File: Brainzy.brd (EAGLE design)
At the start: 80 x 75 mm, 74 parts, among them J7 5.5x2.1mm Barrel, Q1 BSS138, Q2 BSS138, Q3 BSS138, Q4 BSS138, T1 BSS84, T2 BSS84, T3 BSS84, T4 SI2323DS, U1 L293DD, U2 L293DD, U3 HC_05, U4 GY-521MPU6050

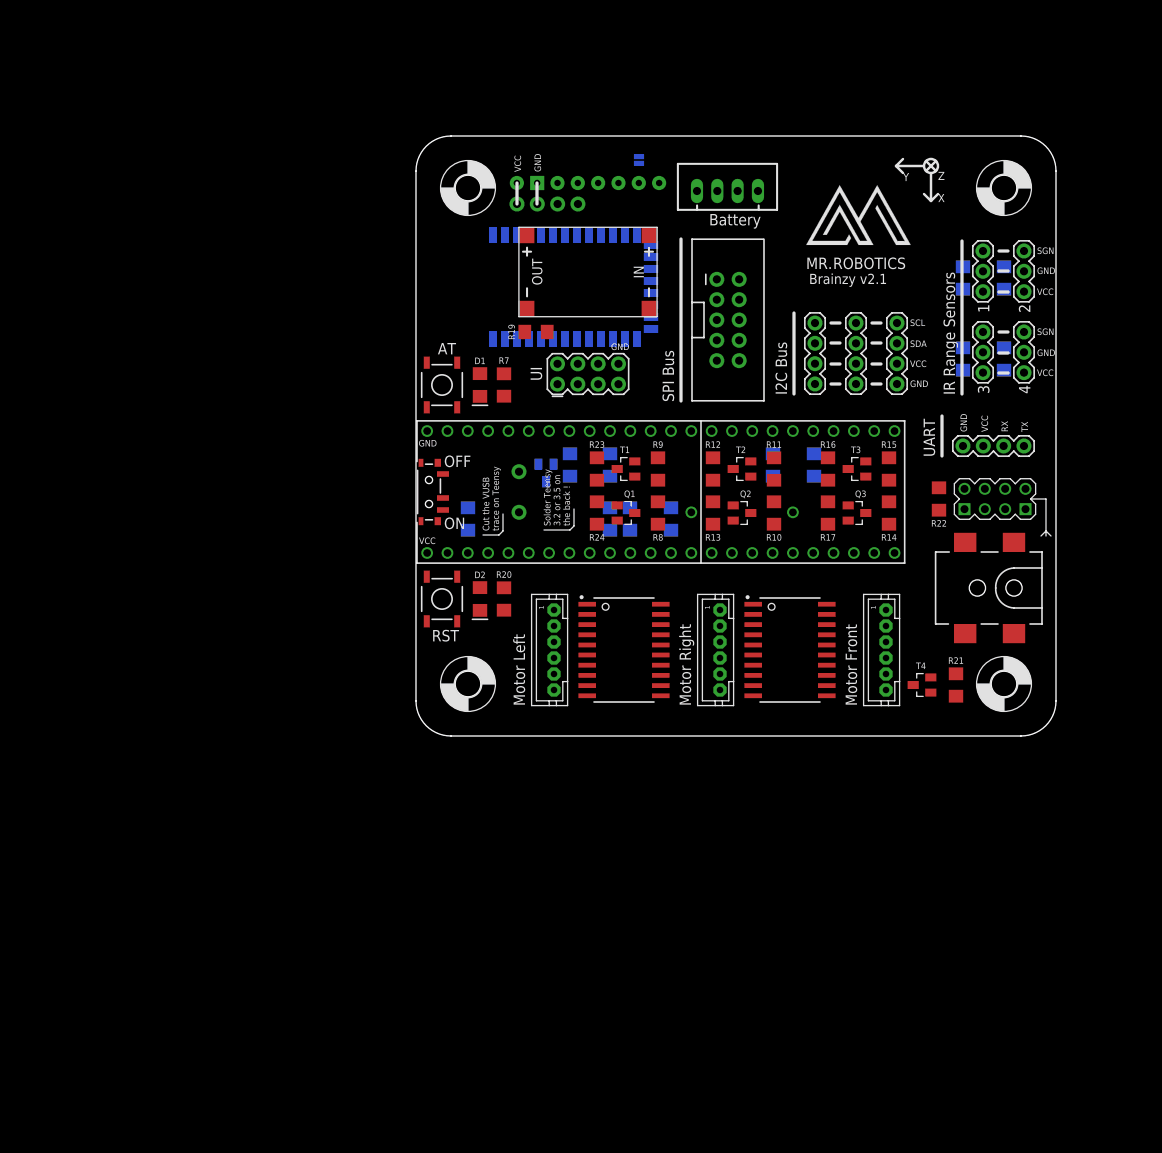
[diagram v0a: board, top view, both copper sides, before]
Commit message: Upload Brainzy v3.0
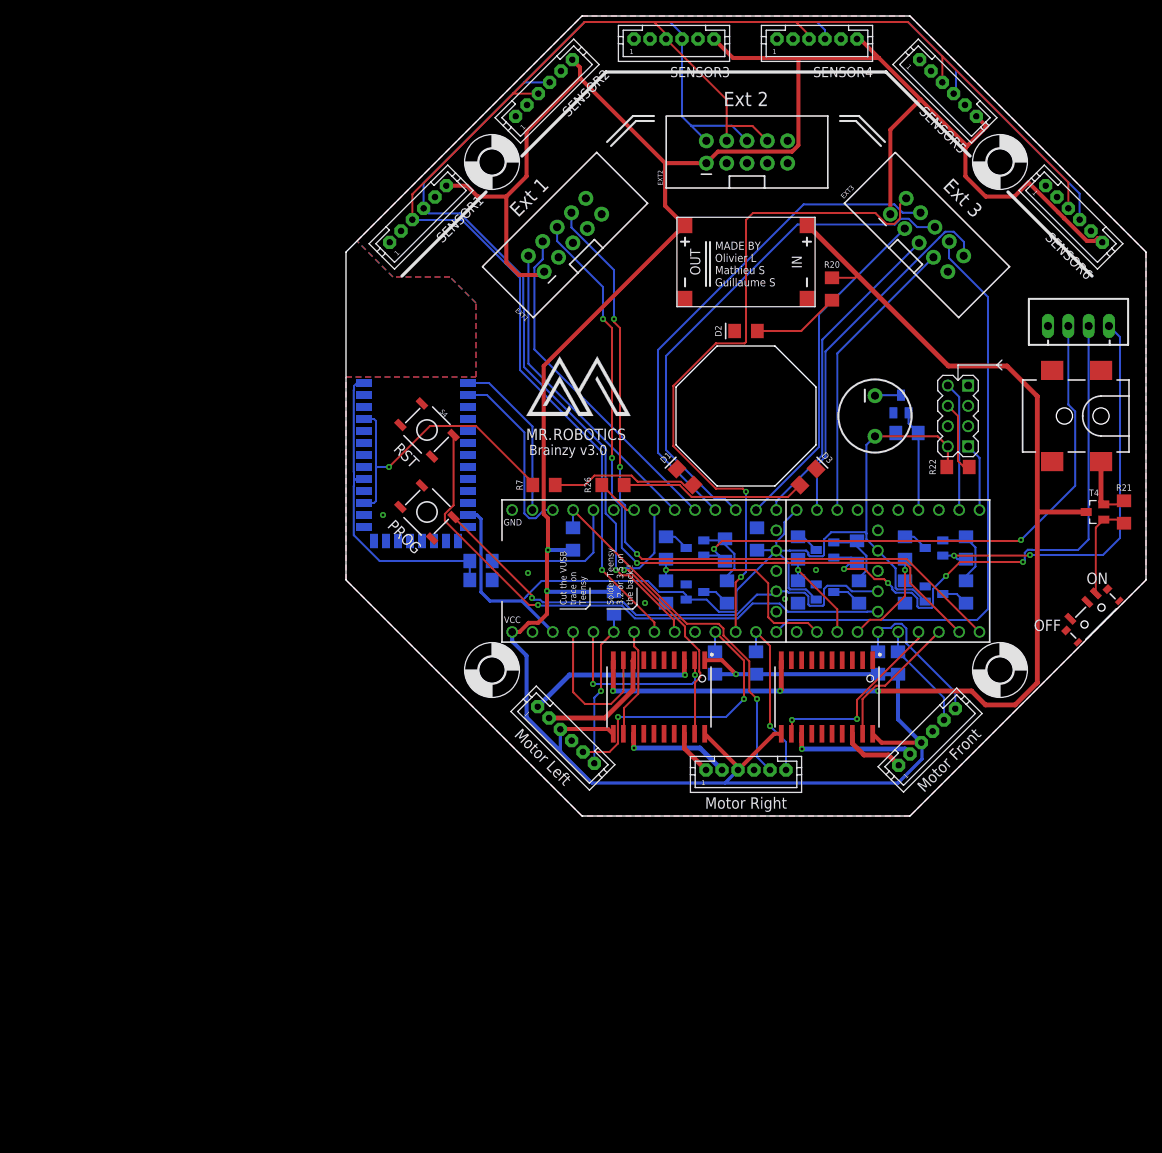
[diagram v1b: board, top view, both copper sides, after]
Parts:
- removed C1, C2, C3, C4: 10uF, SparkFun-Capacitors:1206
- removed EXT_BT: (no value), SparkFun-Connectors:1X04_NO_SILK
- removed H1, H2, H3, H4: MOUNT-HOLE3.2, holes:3,2
- removed I2C1, I2C2, I2C3, UART: (no value), SparkFun-Connectors:1X04
- removed JP1: JUMPER-SMT_2_NO_NO-SILK, SparkFun-Jumpers:SMT-JUMPER_2_NO_NO-SILK
- removed S1: (no value), SparkFun-Switches:TACTILE_SWITCH_SMD_5.2MM
- removed SHARP1, SHARP2, SHARP3, SHARP4: (no value), SparkFun-Connectors:1X03
- removed SPI: (no value), MrRobotics-Connectors:2X5-SHROUDED_LOCK
- removed U$4: LOGO_FR, MrRobotics-Aesthetics:LOGO_FR
- removed U4: GY-521MPU6050, MrRobotics-Modules:GY-521
- removed UI: (no value), SparkFun-Connectors:2X4
- added D3: (no value), SparkFun-LED:FKIT-LED-1206
- added EXT1, EXT2, EXT3: (no value), SparkFun-Connectors:2X5-SHROUDED_LOCK
- added R26, R27: 470, SparkFun-Resistors:1206
- added S4: (no value), SparkFun-Switches:TACTILE_SWITCH_SMD_5.2MM
- added SENSOR1, SENSOR2, SENSOR3, SENSOR4, SENSOR5, SENSOR6: (no value), MrRobotics-Connectors:JST-PH6
- added U$10, U$11, U$8, U$9: (no value), holes:3,3
- added U$12: (no value), MrRobotics-Aesthetics:LOGO_M
- added U$5: (no value), MrRobotics-Aesthetics:M_50MM
- R23: value 470k -> 150k
- R24: value 150k -> 470k
- R7: value 750 -> 470
- U$3: value LOGO -> (none); device MrRobotics-Aesthetics:LOGO_M -> MrRobotics-Aesthetics:LOGO_FR
- U$7: device MrRobotics-Aesthetics:LOGO_BACK_NAME -> MrRobotics-Aesthetics:NAME_50MM
- moved S2 84.4 mm to (84.6, 15.0), turned to 225 degrees
- moved U$3 64.6 mm to (28.1, 0.12), flipped to the bottom
- moved R20 56.4 mm to (52.0, 55.9), turned to 90 degrees
- moved U$7 53.0 mm to (65.8, 51.0)
- moved D2 47.2 mm to (41.2, 50.6), turned to 180 degrees
- moved BATT 47.0 mm to (79.0, 51.2)
- moved BUZZER 45.5 mm to (57.4, 40.0), flipped to the top
- moved Q4 45.2 mm to (60.6, 41.5), turned to 0 degrees
- moved R25 42.3 mm to (61.4, 37.9), turned to 0 degrees
- moved R18 36.2 mm to (42.6, 24.6), turned to 270 degrees
- moved R19 31.8 mm to (8.12, 19.5), flipped to the bottom, turned to 180 degrees
- moved R3 30.8 mm to (42.5, 9.12)
- moved T4 30.6 mm to (84.9, 28.0)
- moved R21 30.1 mm to (88.5, 28.0)
- moved D1 28.1 mm to (33.6, 32.4), turned to 135 degrees
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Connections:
- net N$12 renamed PROG
- removed net BTN_CENTER: U$1.4, UI.5
- removed net BTN_DOWN: U$1.7, UI.4
- removed net BTN_LEFT: U$1.3, UI.3
- removed net BTN_RIGHT: U$1.5, UI.6
- removed net BTN_UP: U$1.2, UI.1
- removed net BT_RST: S3.1, U3.11
- removed net DTR: U3.32
- removed net EXT_RX: U$1.31/A12, UART.3
- removed net EXT_TX: U$1.32/A13, UART.4
- removed net MPU_INT: U$1.26, U4.INT
- removed net N$17: JP1.1, U4.ADO
- removed net SHARP1: SHARP1.1, U$1.38/A19
- removed net SHARP2: SHARP2.1, U$1.37/A18
- removed net SHARP3: SHARP3.1, U$1.35/A16
- removed net SHARP4: SHARP4.1, U$1.36/A17
- new net BT_KEY: R27.2, U$1.3
- new net EXT1_RX: EXT1.2, U$1.7
- new net EXT1_TX: EXT1.4, U$1.8
- new net EXT2_RX: EXT1.6, U$1.34/A15
- new net EXT2_TX: EXT1.8, U$1.33/A14
- new net LED_BUILDIN: R26.1, U$1.5
- new net N$12: D3.A, R26.2
- new net RST: S4.2, U$1.RST_3.5
- net 3.3V: now also U$1.3.3V2, U$1.3.3V3; no longer S1.3
- net 5V: now also EXT1.1, EXT2.1, EXT3.1, SENSOR1.6, SENSOR2.6, SENSOR3.6, SENSOR4.6, SENSOR5.6, SENSOR6.6; no longer C1.1, C2.1, C3.1, C4.1, EXT_BT.1, I2C1.2, I2C2.2, I2C3.2, JP1.2, SHARP1.3, SHARP2.3, SHARP3.3, SHARP4.3, SPI.1, U4.VCC, UART.2, UI.2
- net BATT1: now also U$1.A22; no longer U$1.39/A20
- net BATT3: now also U$1.39/A20; no longer U$1.A22
- net BT_RX: no longer EXT_BT.3
- net BT_TX: no longer EXT_BT.4
- net ENC1_B: now also MOT_LEFT.6, R1.1, U$1.21/A7; no longer U$1.17/A3
- net ENC2_A: now also U$1.2; no longer U$1.8
- net ENC2_B: no longer MOT_LEFT.6, R1.1
- net ENC3_A: now also U$1.37/A18; no longer U$1.27
- net ENC3_B: now also U$1.38/A19; no longer U$1.28
- net GND: now also D3.C, EXT1.9, EXT2.9, EXT3.9, S4.4, SENSOR1.1, SENSOR2.1, SENSOR3.1, SENSOR4.1, SENSOR5.1, SENSOR6.1, U$1.GND2, U$1.GND3; no longer C1.2, C2.2, C3.2, C4.2, EXT_BT.2, I2C1.1, I2C2.1, I2C3.1, S3.3, SHARP1.2, SHARP2.2, SHARP3.2, SHARP4.2, SPI.2, U4.GND, UART.1, UI.8
- net I2C_SCL: now also EXT2.4, EXT2.8, SENSOR1.3, SENSOR2.3, SENSOR3.3, SENSOR4.3, SENSOR5.3, SENSOR6.3; no longer I2C1.4, I2C2.4, I2C3.4, U4.SCL
- net I2C_SDA: now also EXT2.2, EXT2.6, SENSOR1.4, SENSOR2.4, SENSOR3.4, SENSOR4.4, SENSOR5.4, SENSOR6.4; no longer I2C1.3, I2C2.3, I2C3.3, U4.SDA
- net MOT1_1: now also U$1.22/A8, U1.2; no longer U$1.23/A9, U1.9
- net MOT1_2: now also U$1.23/A9, U1.9; no longer U$1.22/A8, U1.2
- net MOT1_OUT1: now also U1.3; no longer U1.8
- net MOT1_OUT2: now also U1.8; no longer U1.3
- net MOT2_1: now also U$1.6, U1.19; no longer U$1.21/A7, U1.12
- net MOT2_2: now also U1.12; no longer U1.19
- net MOT2_OUT1: now also U1.18; no longer U1.13
- net MOT2_OUT2: now also U1.13; no longer U1.18
- net MOT3_1: now also U$1.35/A16, U2.19; no longer U$1.29, U2.12
- net MOT3_2: now also U$1.36/A17, U2.12; no longer U$1.30, U2.19
- net MOT3_OUT1: now also U2.18; no longer U2.13
- net MOT3_OUT2: now also U2.13; no longer U2.18
- net N$18: now also R27.1; no longer S1.1
- net N$8: now also U$1.29; no longer U$1.6
- net SPI_CS1: now also EXT3.2; no longer SPI.4
- net SPI_CS2: now also EXT3.4; no longer SPI.6
- net SPI_CS3: now also EXT3.6; no longer SPI.8
- net SPI_MISO: now also EXT3.5; no longer SPI.7
- net SPI_MOSI: now also EXT3.3; no longer SPI.5
- net SPI_SCK: now also EXT3.8; no longer SPI.3
- net T_CS: now also EXT3.7; no longer SPI.9
- net T_IRQ: now also EXT3.10; no longer SPI.10
- net WIFI_RX: now also U$1.31/A12; no longer U$1.34/A15
- net WIFI_TX: now also U$1.32/A13; no longer U$1.33/A14
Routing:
- net 5V: track 0.00 -> 393.6 mm, vias 0 -> 3
- net I2C_SDA: track 0.00 -> 207.7 mm, vias 0 -> 1
- net I2C_SCL: track 0.00 -> 207.0 mm, vias 0 -> 1
- net 12V: track 0.00 -> 145.5 mm, vias 0 -> 3
- net 3.3V: track 0.00 -> 131.1 mm
- net EXT2_TX: track 0.00 -> 92.9 mm, vias 0 -> 3
- net EXT2_RX: track 0.00 -> 91.1 mm, vias 0 -> 3
- net SPI_CS1: track 0.00 -> 86.9 mm, vias 0 -> 2
- net SPI_SCK: track 0.00 -> 75.6 mm
- net S1: track 0.00 -> 73.8 mm, vias 0 -> 2
- net RST: track 0.00 -> 71.6 mm, vias 0 -> 1
- net S2: track 0.00 -> 70.5 mm, vias 0 -> 4
- net SPI_CS3: track 0.00 -> 64.7 mm
- net SPI_CS2: track 0.00 -> 63.8 mm
- net PROG: track 0.00 -> 63.3 mm, vias 0 -> 1
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- added copper zone on layer 1, net GND
- added copper zone on layer 16, net GND
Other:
- board size 80 x 75 mm -> 100 x 100 mm
- board text added: "Brainzy v3.0"
- board text added: "Ext 1"
- board text added: "Ext 2"
- board text added: "Ext 3"
- board text added: "MADE BY Olivier L Mathieu S Guillaume S"
- board text added: "PROG"
- board text removed: "1"
- board text removed: "2"
- board text removed: "3"
- board text removed: "4"
- board text removed: "AT"
- board text removed: "Battery"
- board text removed: "Brainzy v2.1"
- board text removed: "Guillaume Mathieu Olivier"
- board text removed: "I2C Bus"
- board text removed: "IR Range Sensors"
- board text removed: "RX"
- board text removed: "SCL"
- board text removed: "SDA"
- board text removed: "SGN"
- board text removed: "SPI Bus"
- board text removed: "TX"
- board text removed: "UART"
- board text removed: "UI"
- board text removed: "X"
- board text removed: "Y"
- board text removed: "Z"

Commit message: Upload Brainzy v3.1
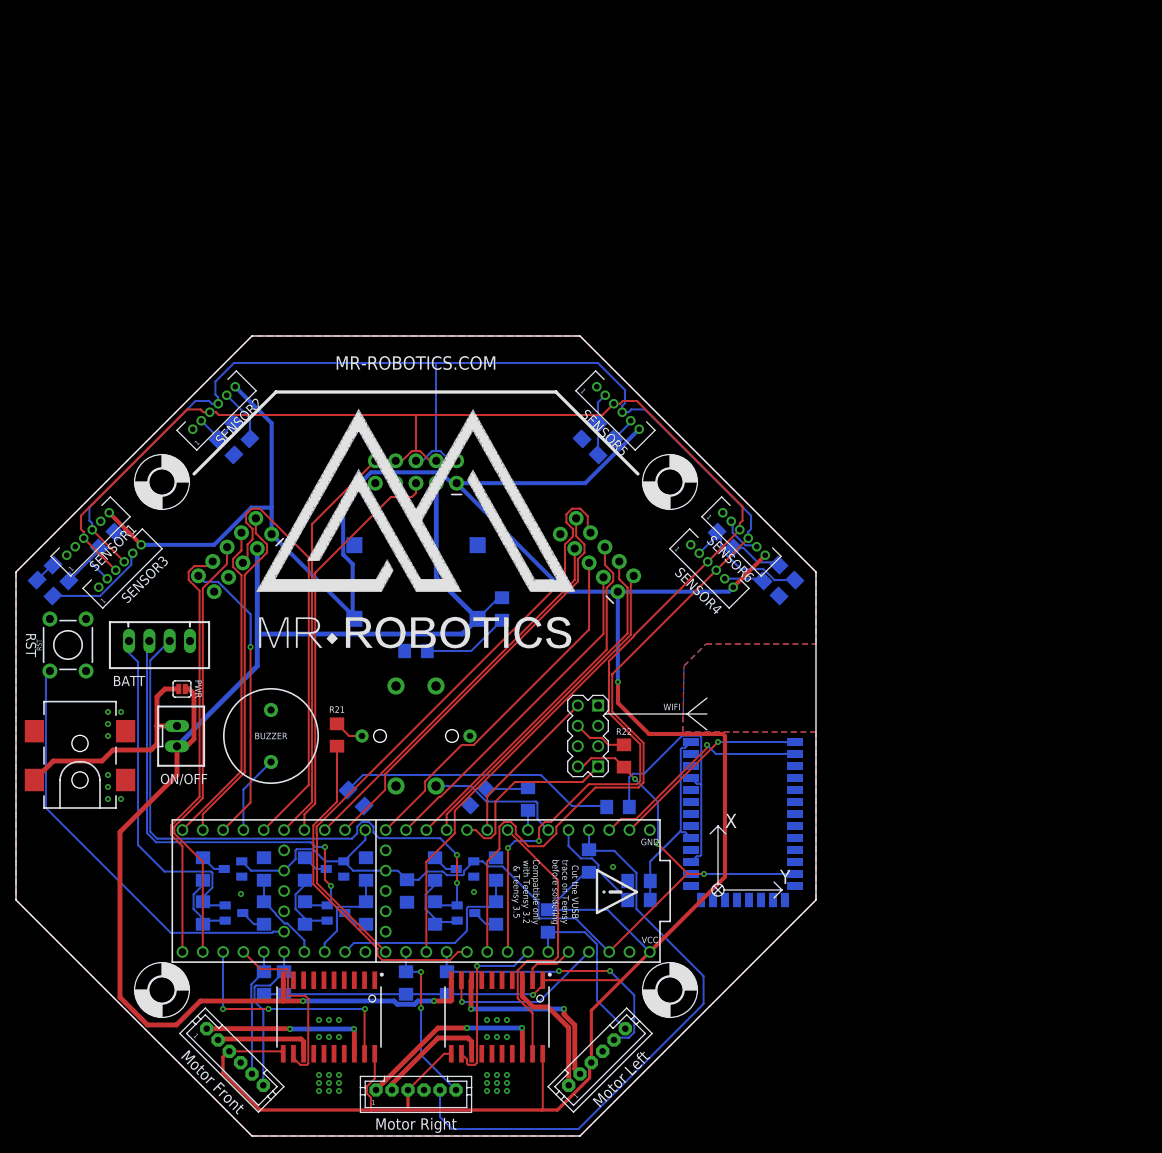
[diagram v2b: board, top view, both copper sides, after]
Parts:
- removed BUZZER: (no value), MrRobotics-Components:BUZZER_5MM
- removed Q4: BSS138, MrRobotics-Transistors:SOT23
- removed S3, S4: (no value), SparkFun-Switches:TACTILE_SWITCH_SMD_5.2MM
- removed T4: SI2323DS, MrRobotics-Transistors:SOT23
- removed U$5: (no value), MrRobotics-Aesthetics:M_50MM
- removed U$7: (no value), MrRobotics-Aesthetics:NAME_50MM
- added LS1: BUZZER-PTH, SparkFun-Electromechanical:BUZZER-12MM
- added ON/OFF: JST-XH-02-PIN-LONG-PAD, MrRobotics-Connectors:JST-XH-02-PACKAGE-LONG-PAD
- added PWR: JUMPER-SMT_2_NO_SILK, SparkFun-Jumpers:SMT-JUMPER_2_NO_SILK
- added R28, R29, R32, R33, R36: 150k, SparkFun-Resistors:1206
- added R30, R31, R34, R35: 470k, SparkFun-Resistors:1206
- added RST: MOMENTARY-SWITCH-SPST-PTH-6.0MM, SparkFun-Switches:TACTILE_SWITCH_PTH_6.0MM
- added U$13: (no value), MrRobotics-Aesthetics:NAME_40MM
- added U$4: (no value), MrRobotics-Aesthetics:M_40MM
- R21: value 470k -> 470
- S2: value (none) -> MOMENTARY-SWITCH-SPST-LED-PTH-12MM; device SparkFun-Switches:SWITCH_SPST_SMD_A -> SparkFun-Switches:TACTILE_SWITCH_LED_PTH_12MM
- SENSOR1, SENSOR2, SENSOR3, SENSOR4, SENSOR5, SENSOR6: device MrRobotics-Connectors:JST-PH6 -> MrRobotics-Connectors:JST-ZH6
- U$1: value TEENSY_3.5-3.2INV -> TEENSY_3.5-3.2; device MrRobotics-Boards:TEENSY_3.5-3.2_INV -> MrRobotics-Boards:TEENSY_3.5-3.2
- moved J7 135.5 mm to (-42.0, -5.50), turned to 90 degrees
- moved BATT 114.2 mm to (-28.2, 11.9), turned to 180 degrees
- moved R15 105.7 mm to (-26.6, -22.1), turned to 90 degrees
- moved R21 102.2 mm to (-9.88, 0.12), turned to 90 degrees
- moved R14 101.5 mm to (-26.6, -16.6), turned to 270 degrees
- moved T3 98.7 mm to (-22.8, -22.1), turned to 90 degrees
- moved SENSOR3 95.6 mm to (-37.0, 21.2), turned to 225 degrees
- moved MOT_FRONT 95.3 mm to (-22.6, -40.1), turned to 135 degrees
- moved Q3 94.1 mm to (-22.9, -16.6), turned to 270 degrees
- moved R16 92.2 mm to (-19.0, -22.1), turned to 270 degrees
- moved R6 88.8 mm to (-19.0, -30.9)
- moved R17 87.3 mm to (-19.0, -16.6), turned to 270 degrees
- moved S2 85.9 mm to (0.00, 0.00), flipped to the bottom, turned to 270 degrees
- moved R5 84.3 mm to (-16.5, -30.9)
- moved R11 82.4 mm to (-13.9, -22.1), turned to 90 degrees
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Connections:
- net EXT2_RX renamed RX5
- net EXT2_TX renamed TX5
- net LED_BUILDIN renamed LED_BUILTIN
- net T_CS renamed D5
- net T_IRQ renamed D6
- removed net EXT1_RX: EXT1.2, U$1.7
- removed net EXT1_TX: EXT1.4, U$1.8
- removed net PROG: S3.2, U$1.PGM_3.2, U$1.PGM_3.5
- new net BTN_PROG: S2.4, U$1.4
- new net D1: EXT1.5, U$1.28
- new net D2: EXT1.10, U$1.30
- new net D3: EXT2.5, U$1.26
- new net D4: EXT2.10, U$1.27
- new net LED_BTN_PROG: R21.1, U$1.17/A3
- new net N$17: SENSOR6.2, SENSOR6.5
- new net N$21: R28.1, SENSOR4.5
- new net N$22: R31.2, R32.2, SENSOR5.2
- new net N$23: R32.1, SENSOR5.5
- new net N$24: R29.2, R30.2, SENSOR2.2
- new net N$25: R30.1, SENSOR2.5
- new net N$26: R33.2, R35.2
- new net N$27: R34.2, R35.1, SENSOR3.2
- new net N$28: R33.1, SENSOR3.5
- new net N$29: R28.2, R36.2
- new net RX4: EXT1.2, U$1.31/A12
- new net TX4: EXT1.4, U$1.32/A13
- new net WIFI_RST: U$6.C2
- net 12V: now also EXT1.3, EXT2.3, ON/OFF.2, PWR.2; no longer T4.3
- net 3.3V: no longer BUZZER.2
- net GND: now also EXT1.7, EXT2.7, LS1.-, R25.1, R29.1, R31.1, R34.1, RST.3, S2.C, SENSOR1.2; no longer Q4.2, R25.2, S2.3, S3.4, S4.4
- net N$15: now also ON/OFF.1, PWR.1; no longer R21.1, T4.2
- net N$16: now also S2.A; no longer S2.1, T4.1
- net N$20: now also R25.2, R36.1, SENSOR4.2; no longer BUZZER.1, Q4.3
- net N$8: now also LS1.+; no longer Q4.1, R25.1
- net RST: now also RST.1; no longer S4.2
- net WIFI_RX: now also U$1.7; no longer U$1.31/A12
- net WIFI_TX: now also U$1.8; no longer U$1.32/A13
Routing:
- net PROG: track 63.3 -> 0.00 mm, vias 1 -> 0
- net D1: track 0.00 -> 54.0 mm
- net D4: track 0.00 -> 50.9 mm
- net D3: track 0.00 -> 50.7 mm
- net RX4: track 0.00 -> 42.9 mm
- net LED_BTN_PROG: track 0.00 -> 42.5 mm
- net EXT1_TX: track 42.3 -> 0.00 mm
- net TX4: track 0.00 -> 41.1 mm
- net EXT1_RX: track 39.4 -> 0.00 mm
- net TX5: track 92.9 -> 53.7 mm, vias 3 -> 0
- net D2: track 0.00 -> 36.9 mm, vias 0 -> 1
- net RX5: track 91.1 -> 54.8 mm, vias 3 -> 0
- net SPI_CS1: track 86.9 -> 57.8 mm, vias 2 -> 0
- net 12V: track 145.5 -> 173.9 mm, vias 3 -> 2
- net ENC2_A: track 47.2 -> 72.9 mm, vias 1 -> 0
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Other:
- outline, holes or cut-outs redrawn
- board text added: "BATT"
- board text added: "BLUETOOTH"
- board text added: "BUZZER"
- board text added: "Brainzy v3.1"
- board text added: "CO-FOUNDERS Olivier L Mathieu S Guillaume S"
- board text added: "Cut the VUSB trace on Teensy before soldering Compatible only with Teensy 3.2 & Teensy 3.5"
- board text added: "I2C"
- board text added: "ON/OFF"
- board text added: "SPI"
- board text added: "UART"
- board text added: "WIFI"
- board text added: "X"
- board text added: "Y"
- board text removed: "Brainzy v3.0"
- board text removed: "Cut the VUSB trace on Teensy"
- board text removed: "Ext 1"
- board text removed: "Ext 2"
- board text removed: "Ext 3"
- board text removed: "MADE BY Olivier L Mathieu S Guillaume S"
- board text removed: "OFF"
- board text removed: "ON"
- board text removed: "PROG"
- board text removed: "Solder Teensy 3.2 or 3.5 on the back !"
